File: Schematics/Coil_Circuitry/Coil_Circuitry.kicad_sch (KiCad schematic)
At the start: 15 parts, among them J1 Conn_01x04_Pin, Q1 PMOS, Q2 NMOS, SW2 Manual, U1 MOUDLE-SEEEDUINO-XIAO-ESP32C3

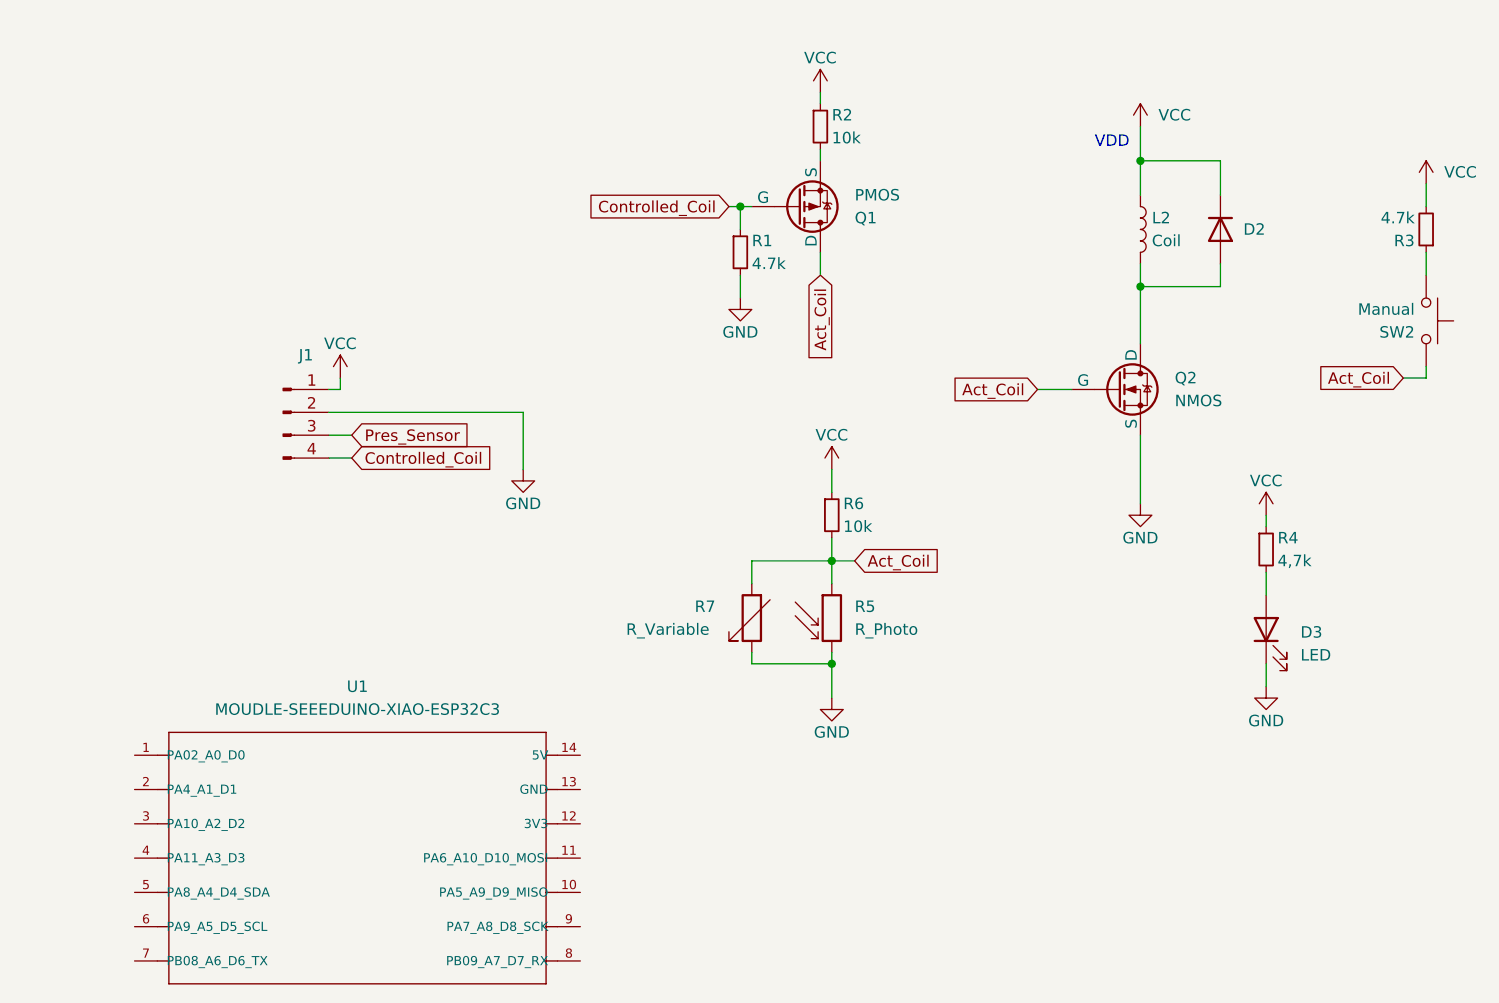
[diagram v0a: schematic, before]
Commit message: fegcv
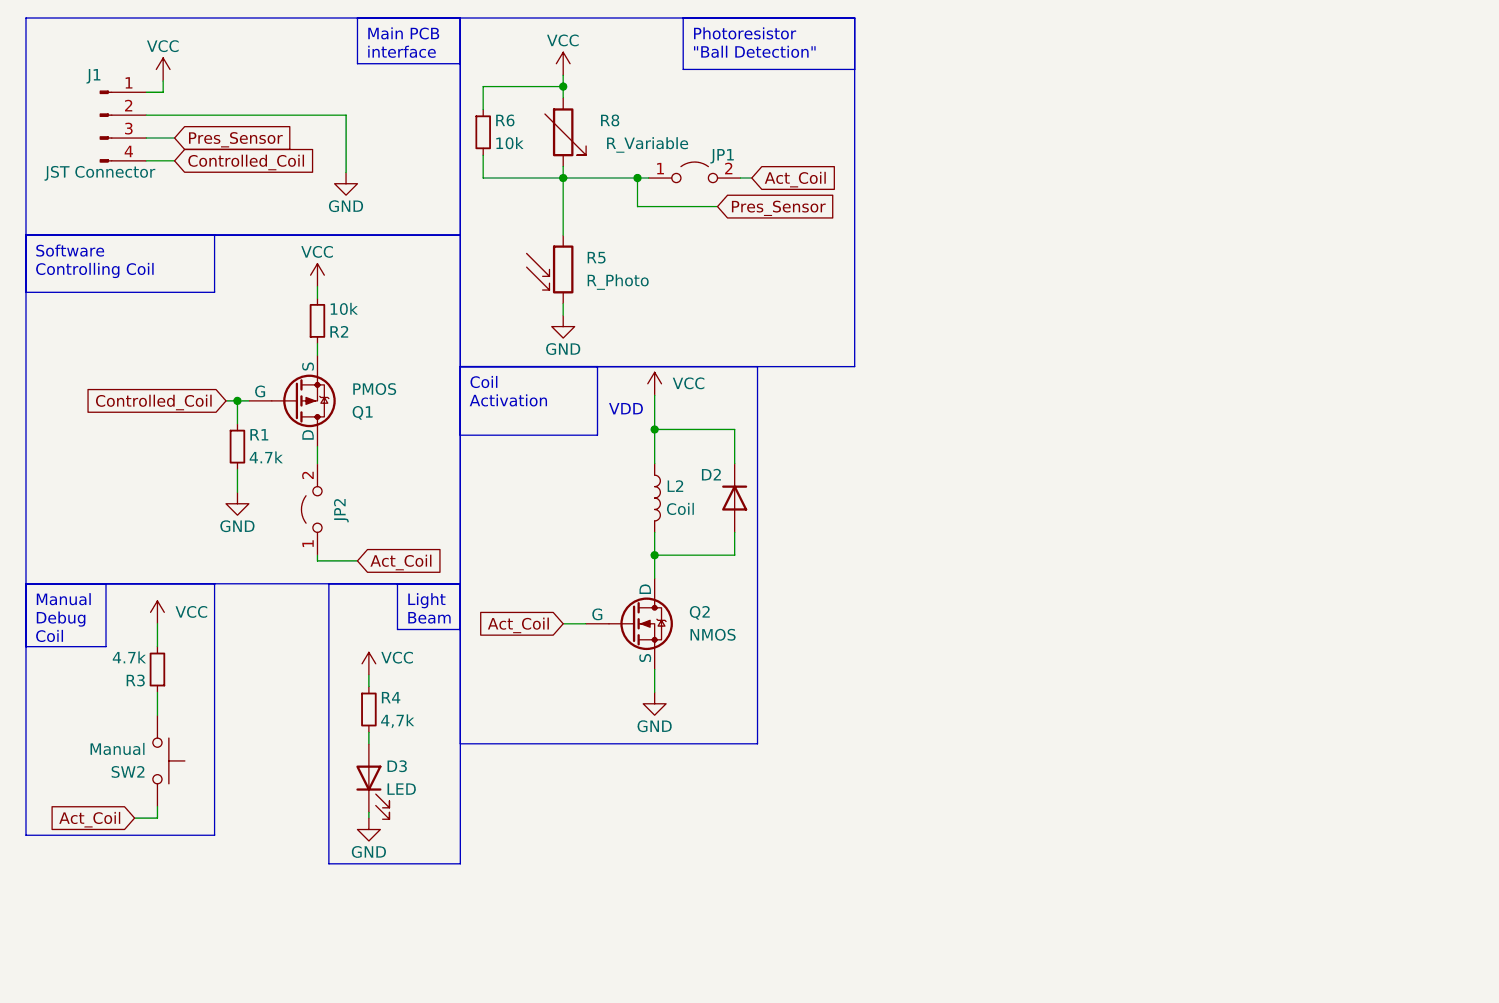
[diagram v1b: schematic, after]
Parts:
- removed R7: R_Variable, symbol Device:R_Variable
- removed U1: MOUDLE-SEEEDUINO-XIAO-ESP32C3, MOUDLE14P-SMD-2.54-21X17.8MM, symbol MOUDLE-SEEEDUINO-XIAO-ESP32C3:MOUDLE-SEEEDUINO-XIAO-ESP32C3
- added JP1: Jumper_2_Open, symbol Jumper:Jumper_2_Open
- added JP2: Jumper_2_Open, Connector_PinHeader_1.00mm:PinHeader_1x02_P1.00mm_Vertical, symbol Jumper:Jumper_2_Open
- added R8: R_Variable, symbol Device:R_Variable
- J1: footprint (none) -> Connector_JST:JST_XH_B4B-XH-A_1x04_P2.50mm_Vertical; Note (none) -> JST Connector
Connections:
- net Act_Coil: now also JP1.2 (B), JP2.1 (A); no longer Q1.1 (D), R5.1, R6.2
- net Pres_Sensor: now also R5.1, R6.2, JP1.1 (A), R8.1
- net VCC: now also R2.2, R8.2; no longer R2.1
- net at Q1.3 (S): now also R2.1; no longer R2.2
- new net: JP2.2 (B), Q1.1 (D)
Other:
- moved on the sheet: D2, D3, L2, Q1, Q2, R1, R2, R3, R4, R5, R6, SW2
